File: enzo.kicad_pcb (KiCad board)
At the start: 2 copper layers, 118 x 95.1 mm, 61 parts, among them SW1 SW_Push, SW10 SW_Push, SW11 SW_Push, SW12 SW_Push, SW13 SW_Push, SW14 SW_Push, SW15 SW_Push, SW16 SW_Push, SW17 locked, SW2 SW_Push, SW3 SW_Push, SW4 SW_Push, SW5 SW_Push, SW6 SW_Push, SW7 SW_Push, SW8 SW_Push, SW9 SW_Push

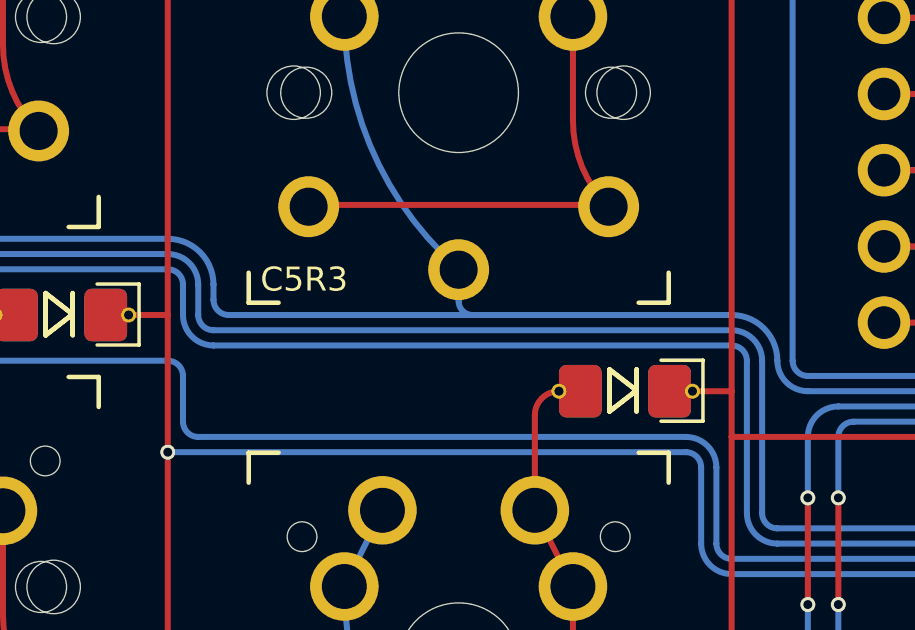
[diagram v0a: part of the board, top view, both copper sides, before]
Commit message: Fix traces
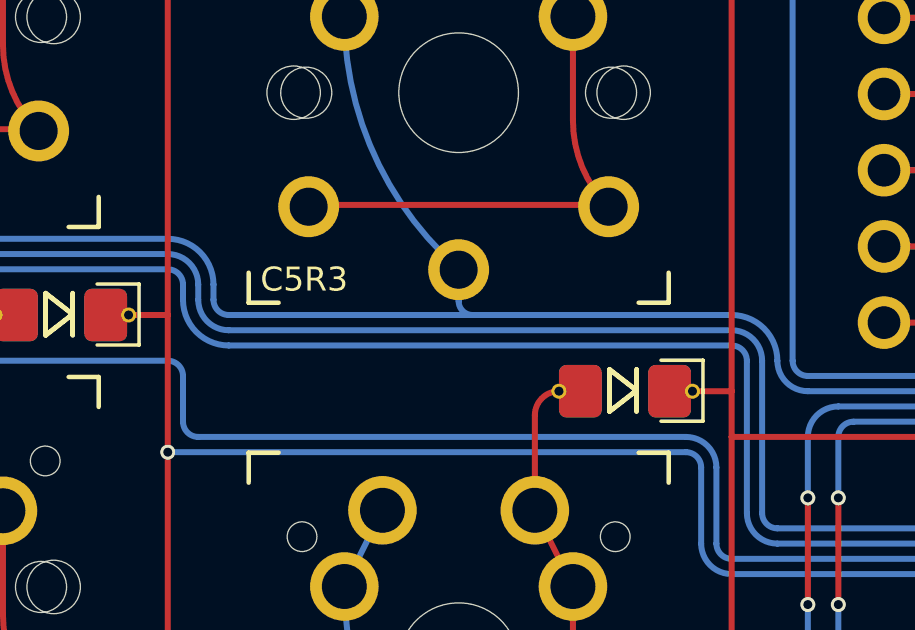
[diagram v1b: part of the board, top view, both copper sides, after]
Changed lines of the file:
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@@
   (arc (start 98.552 107.696) (mid 98.91121 107.54721) (end 99.06 107.188) (width 0.2) (layer "F.Cu") (net 22))
   (arc (start 184.032387 84.074) (mid 184.255572 84.612815) (end 184.794387 84.836) (width 0.2) (layer "F.Cu") (net 22))
+  (segment (start 138.684 88.392) (end 138.684 90.932) (width 0.2) (layer "B.Cu") (net 22))
+  (segment (start 158.496 94.488) (end 175.26 94.488) (width 0.2) (layer "B.Cu") (net 22))
+  (segment (start 119.38 92.456) (end 119.38 88.392) (width 0.2) (layer "B.Cu") (net 22))
+  (segment (start 191.008 84.836) (end 191.114387 84.836) (width 0.2) (layer "B.Cu") (net 22))
   (segment (start 176.276 95.504) (end 176.276 100.584) (width 0.2) (layer "B.Cu") (net 22))
-  (segment (start 119.38 92.456) (end 119.38 88.392) (width 0.2) (layer "B.Cu") (net 22))
-  (segment (start 157.48 92.964) (end 157.48 93.98) (width 0.2) (layer "B.Cu") (net 22))
+  (segment (start 188.468 100.584) (end 188.468 86.36) (width 0.2) (layer "B.Cu") (net 22))
+  (segment (start 157.48 92.964) (end 157.48 93.472) (width 0.2) (layer "B.Cu") (net 22))
   (segment (start 101.6 93.472) (end 118.364 93.472) (width 0.2) (layer "B.Cu") (net 22))
-  (segment (start 157.988 94.488) (end 175.26 94.488) (width 0.2) (layer "B.Cu") (net 22))
+  (segment (start 189.992 84.836) (end 191.008 84.836) (width 0.2) (layer "B.Cu") (net 22))
   (segment (start 176.784 101.092) (end 187.96 101.092) (width 0.2) (layer "B.Cu") (net 22))
-  (segment (start 189.992 84.836) (end 191.008 84.836) (width 0.2) (layer "B.Cu") (net 22))
   (segment (start 120.396 87.376) (end 137.668 87.376) (width 0.2) (layer "B.Cu") (net 22))
-  (segment (start 191.008 84.836) (end 191.114387 84.836) (width 0.2) (layer "B.Cu") (net 22))
-  (segment (start 188.468 100.584) (end 188.468 86.36) (width 0.2) (layer "B.Cu") (net 22))
-  (segment (start 138.684 88.392) (end 138.684 90.932) (width 0.2) (layer "B.Cu") (net 22))
   (segment (start 139.7 91.948) (end 156.464 91.948) (width 0.2) (layer "B.Cu") (net 22))
-  (arc (start 156.464 91.948) (mid 157.18242 92.24558) (end 157.48 92.964) (width 0.2) (layer "B.Cu") (net 22))
-  (arc (start 191.114387 84.836) (mid 191.653202 84.612815) (end 191.876387 84.074) (width 0.2) (layer "B.Cu") (net 22))
-  (arc (start 188.468 86.36) (mid 188.914369 85.282369) (end 189.992 84.836) (width 0.2) (layer "B.Cu") (net 22))
-  (arc (start 175.26 94.488) (mid 175.97842 94.78558) (end 176.276 95.504) (width 0.2) (layer "B.Cu") (net 22))
-  (arc (start 119.38 88.392) (mid 119.67758 87.67358) (end 120.396 87.376) (width 0.2) (layer "B.Cu") (net 22))
-  (arc (start 176.276 100.584) (mid 176.42479 100.94321) (end 176.784 101.092) (width 0.2) (layer "B.Cu") (net 22))
+  (arc (start 101.092 93.98) (mid 101.24079 93.62079) (end 101.6 93.472) (width 0.2) (layer "B.Cu") (net 22))
   (arc (start 138.684 90.932) (mid 138.98158 91.65042) (end 139.7 91.948) (width 0.2) (layer "B.Cu") (net 22))
   (arc (start 137.668 87.376) (mid 138.38642 87.67358) (end 138.684 88.392) (width 0.2) (layer "B.Cu") (net 22))
+  (arc (start 119.38 88.392) (mid 119.67758 87.67358) (end 120.396 87.376) (width 0.2) (layer "B.Cu") (net 22))
+  (arc (start 157.48 93.472) (mid 157.77758 94.19042) (end 158.496 94.488) (width 0.2) (layer "B.Cu") (net 22))
+  (arc (start 191.114387 84.836) (mid 191.653202 84.612815) (end 191.876387 84.074) (width 0.2) (layer "B.Cu") (net 22))
+  (arc (start 118.364 93.472) (mid 119.08242 93.17442) (end 119.38 92.456) (width 0.2) (layer "B.Cu") (net 22))
+  (arc (start 156.464 91.948) (mid 157.18242 92.24558) (end 157.48 92.964) (width 0.2) (layer "B.Cu") (net 22))
+  (arc (start 175.26 94.488) (mid 175.97842 94.78558) (end 176.276 95.504) (width 0.2) (layer "B.Cu") (net 22))
   (arc (start 187.96 101.092) (mid 188.31921 100.94321) (end 188.468 100.584) (width 0.2) (layer "B.Cu") (net 22))
-  (arc (start 157.48 93.98) (mid 157.62879 94.33921) (end 157.988 94.488) (width 0.2) (layer "B.Cu") (net 22))
-  (arc (start 101.092 93.98) (mid 101.24079 93.62079) (end 101.6 93.472) (width 0.2) (layer "B.Cu") (net 22))
-  (arc (start 118.364 93.472) (mid 119.08242 93.17442) (end 119.38 92.456) (width 0.2) (layer "B.Cu") (net 22))
+  (arc (start 188.468 86.36) (mid 188.914369 85.282369) (end 189.992 84.836) (width 0.2) (layer "B.Cu") (net 22))
+  (arc (start 176.276 100.584) (mid 176.42479 100.94321) (end 176.784 101.092) (width 0.2) (layer "B.Cu") (net 22))
   (segment (start 117.058 76.708) (end 118.364 76.708) (width 0.2) (layer "F.Cu") (net 23))
   (segment (start 184.796453 87.376) (end 191.008 87.376) (width 0.2) (layer "F.Cu") (net 23))
@@
   (arc (start 184.034453 86.614) (mid 184.257638 87.152815) (end 184.796453 87.376) (width 0.2) (layer "F.Cu") (net 23))
   (arc (start 117.856 95.504) (mid 118.21521 95.35521) (end 118.364 94.996) (width 0.2) (layer "F.Cu") (net 23))
-  (segment (start 157.988 94.996) (end 175.26 94.996) (width 0.2) (layer "B.Cu") (net 23))
+  (segment (start 139.7 92.456) (end 156.464 92.456) (width 0.2) (layer "B.Cu") (net 23))
+  (segment (start 191.116453 87.376) (end 191.008 87.376) (width 0.2) (layer "B.Cu") (net 23))
+  (segment (start 119.888 94.488) (end 119.888 88.392) (width 0.2) (layer "B.Cu") (net 23))
+  (segment (start 158.496 94.996) (end 175.26 94.996) (width 0.2) (layer "B.Cu") (net 23))
+  (segment (start 156.972 92.964) (end 156.972 93.472) (width 0.2) (layer "B.Cu") (net 23))
+  (segment (start 176.784 101.6) (end 187.96 101.6) (width 0.2) (layer "B.Cu") (net 23))
+  (segment (start 188.976 100.584) (end 188.976 88.9) (width 0.2) (layer "B.Cu") (net 23))
   (segment (start 120.396 87.884) (end 137.668 87.884) (width 0.2) (layer "B.Cu") (net 23))
-  (segment (start 156.972 92.964) (end 156.972 93.98) (width 0.2) (layer "B.Cu") (net 23))
-  (segment (start 191.116453 87.376) (end 191.008 87.376) (width 0.2) (layer "B.Cu") (net 23))
+  (segment (start 175.768 95.504) (end 175.768 100.584) (width 0.2) (layer "B.Cu") (net 23))
   (segment (start 190.5 87.376) (end 191.008 87.376) (width 0.2) (layer "B.Cu") (net 23))
-  (segment (start 119.888 94.488) (end 119.888 88.392) (width 0.2) (layer "B.Cu") (net 23))
-  (segment (start 139.7 92.456) (end 156.464 92.456) (width 0.2) (layer "B.Cu") (net 23))
-  (segment (start 175.768 95.504) (end 175.768 100.584) (width 0.2) (layer "B.Cu") (net 23))
-  (segment (start 188.976 100.584) (end 188.976 88.9) (width 0.2) (layer "B.Cu") (net 23))
+  (segment (start 138.176 88.392) (end 138.176 90.932) (width 0.2) (layer "B.Cu") (net 23))
   (segment (start 117.058 95.504) (end 118.872 95.504) (width 0.2) (layer "B.Cu") (net 23))
-  (segment (start 138.176 88.392) (end 138.176 90.932) (width 0.2) (layer "B.Cu") (net 23))
-  (segment (start 176.784 101.6) (end 187.96 101.6) (width 0.2) (layer "B.Cu") (net 23))
   (arc (start 188.976 88.9) (mid 189.422369 87.822369) (end 190.5 87.376) (width 0.2) (layer "B.Cu") (net 23))
   (arc (start 119.888 88.392) (mid 120.03679 88.03279) (end 120.396 87.884) (width 0.2) (layer "B.Cu") (net 23))
+  (arc (start 138.176 90.932) (mid 138.622369 92.009631) (end 139.7 92.456) (width 0.2) (layer "B.Cu") (net 23))
+  (arc (start 187.96 101.6) (mid 188.67842 101.30242) (end 188.976 100.584) (width 0.2) (layer "B.Cu") (net 23))
+  (arc (start 156.972 93.472) (mid 157.418369 94.549631) (end 158.496 94.996) (width 0.2) (layer "B.Cu") (net 23))
+  (arc (start 137.668 87.884) (mid 138.02721 88.03279) (end 138.176 88.392) (width 0.2) (layer "B.Cu") (net 23))
+  (arc (start 191.878453 86.614) (mid 191.655268 87.152815) (end 191.116453 87.376) (width 0.2) (layer "B.Cu") (net 23))
+  (arc (start 118.872 95.504) (mid 119.59042 95.20642) (end 119.888 94.488) (width 0.2) (layer "B.Cu") (net 23))
+  (arc (start 175.768 100.584) (mid 176.06558 101.30242) (end 176.784 101.6) (width 0.2) (layer "B.Cu") (net 23))
+  (arc (start 175.26 94.996) (mid 175.61921 95.14479) (end 175.768 95.504) (width 0.2) (layer "B.Cu") (net 23))
   (arc (start 156.464 92.456) (mid 156.82321 92.60479) (end 156.972 92.964) (width 0.2) (layer "B.Cu") (net 23))
-  (arc (start 175.26 94.996) (mid 175.61921 95.14479) (end 175.768 95.504) (width 0.2) (layer "B.Cu") (net 23))
-  (arc (start 175.768 100.584) (mid 176.06558 101.30242) (end 176.784 101.6) (width 0.2) (layer "B.Cu") (net 23))
-  (arc (start 138.176 90.932) (mid 138.622369 92.009631) (end 139.7 92.456) (width 0.2) (layer "B.Cu") (net 23))
-  (arc (start 156.972 93.98) (mid 157.26958 94.69842) (end 157.988 94.996) (width 0.2) (layer "B.Cu") (net 23))
-  (arc (start 191.878453 86.614) (mid 191.655268 87.152815) (end 191.116453 87.376) (width 0.2) (layer "B.Cu") (net 23))
-  (arc (start 187.96 101.6) (mid 188.67842 101.30242) (end 188.976 100.584) (width 0.2) (layer "B.Cu") (net 23))
-  (arc (start 118.872 95.504) (mid 119.59042 95.20642) (end 119.888 94.488) (width 0.2) (layer "B.Cu") (net 23))
-  (arc (start 137.668 87.884) (mid 138.02721 88.03279) (end 138.176 88.392) (width 0.2) (layer "B.Cu") (net 23))
   (segment (start 137.16 63.2465) (end 137.16 70.612) (width 0.2) (layer "F.Cu") (net 24))
   (segment (start 135.854 89.408) (end 136.652 89.408) (width 0.2) (layer "F.Cu") (net 24))
